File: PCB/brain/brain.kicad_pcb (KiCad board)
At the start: 4 copper layers, 100 x 115 mm, 225 parts, among them J1 Screw_Terminal_01x02, J10 Conn_01x12, J11 Conn_01x04, J12 BAT, J13 Conn_01x05, J14 Conn_01x02, J2 Conn_01x04, J3 RJ45_Hanrun_HR911105A_Horizon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, J4 Conn_01x04, J5 Conn_01x04, J6 Conn_01x04, J7 Conn_01x06, J8 Conn_01x06, J9 Motor, Q1 CSD17577Q3A, Q2 CSD17577Q3A, U1 ESP32-S3-WROOM-1, U10 MAX17049G+T10, U11 AP64501SP-13, U12 AP63205WU, U14 AP63203WU, U2 TMC2209-LA, U3 W5500, U4 MAX98357A, U5 TPD2E2U06DCK, U7 R5460N214AF-TR-FE, U8 CH221K, U9 BQ25792, Y1 25MHz

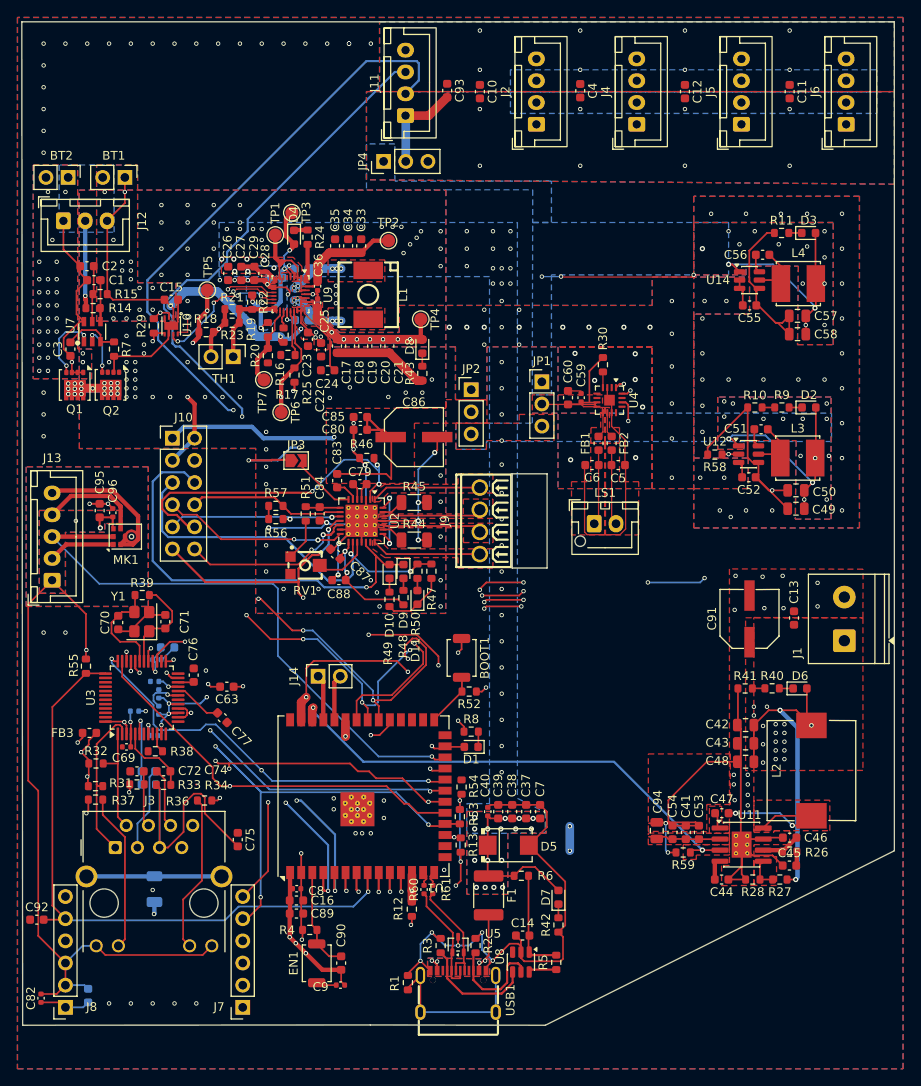
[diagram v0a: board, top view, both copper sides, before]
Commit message: DRC
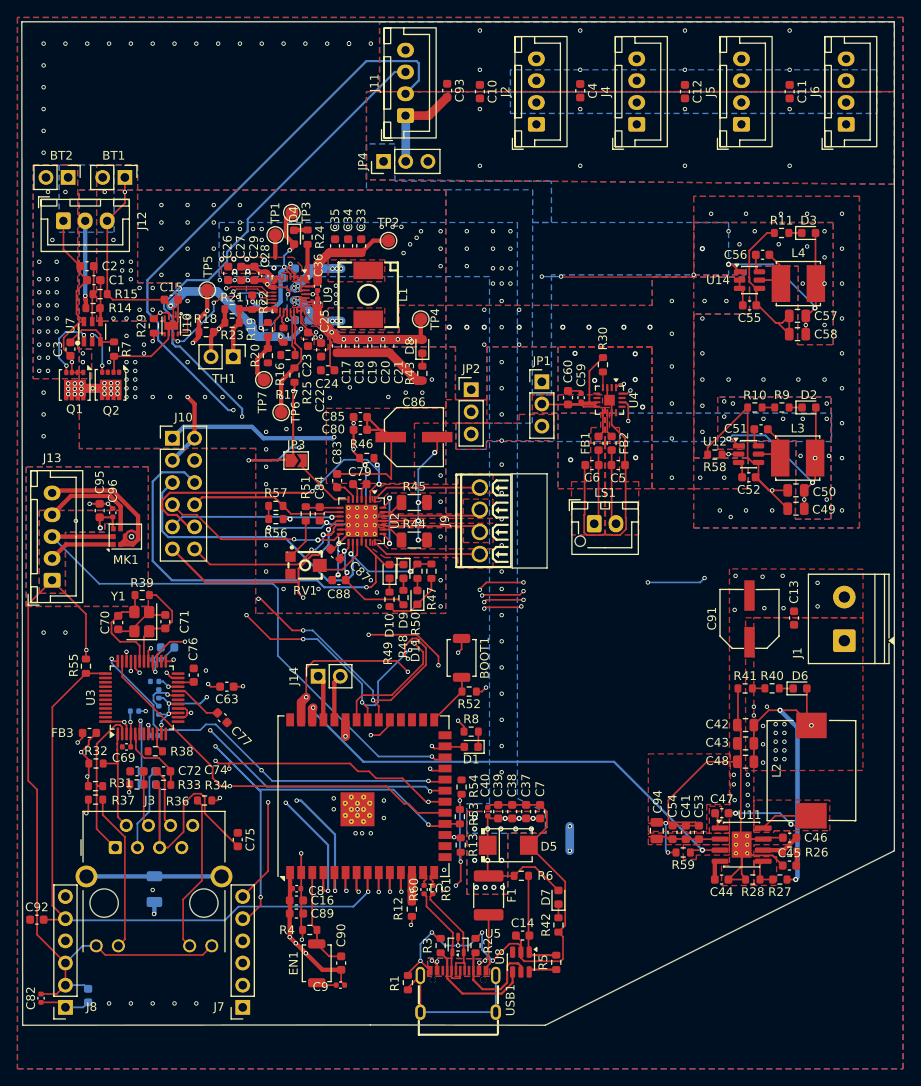
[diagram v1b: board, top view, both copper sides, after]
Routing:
- net +3.3V: track 238.6 -> 246.9 mm
- net VBUS: track 37.5 -> 30.8 mm
- net Net-(U9-BTST1): track 2.61 -> 3.15 mm
- net GND: track 402.7 -> 402.9 mm, vias 202 -> 204
